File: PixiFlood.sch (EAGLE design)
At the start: 36 parts, among them IC1 WS2811-SOP8, IC2 78L05Z, T1 2N3904, T2 2N3904, T3 2N3904, U1 PT4115B89E, U2 PT4115B89E, U3 PT4115B89E, X2 22-23-2041

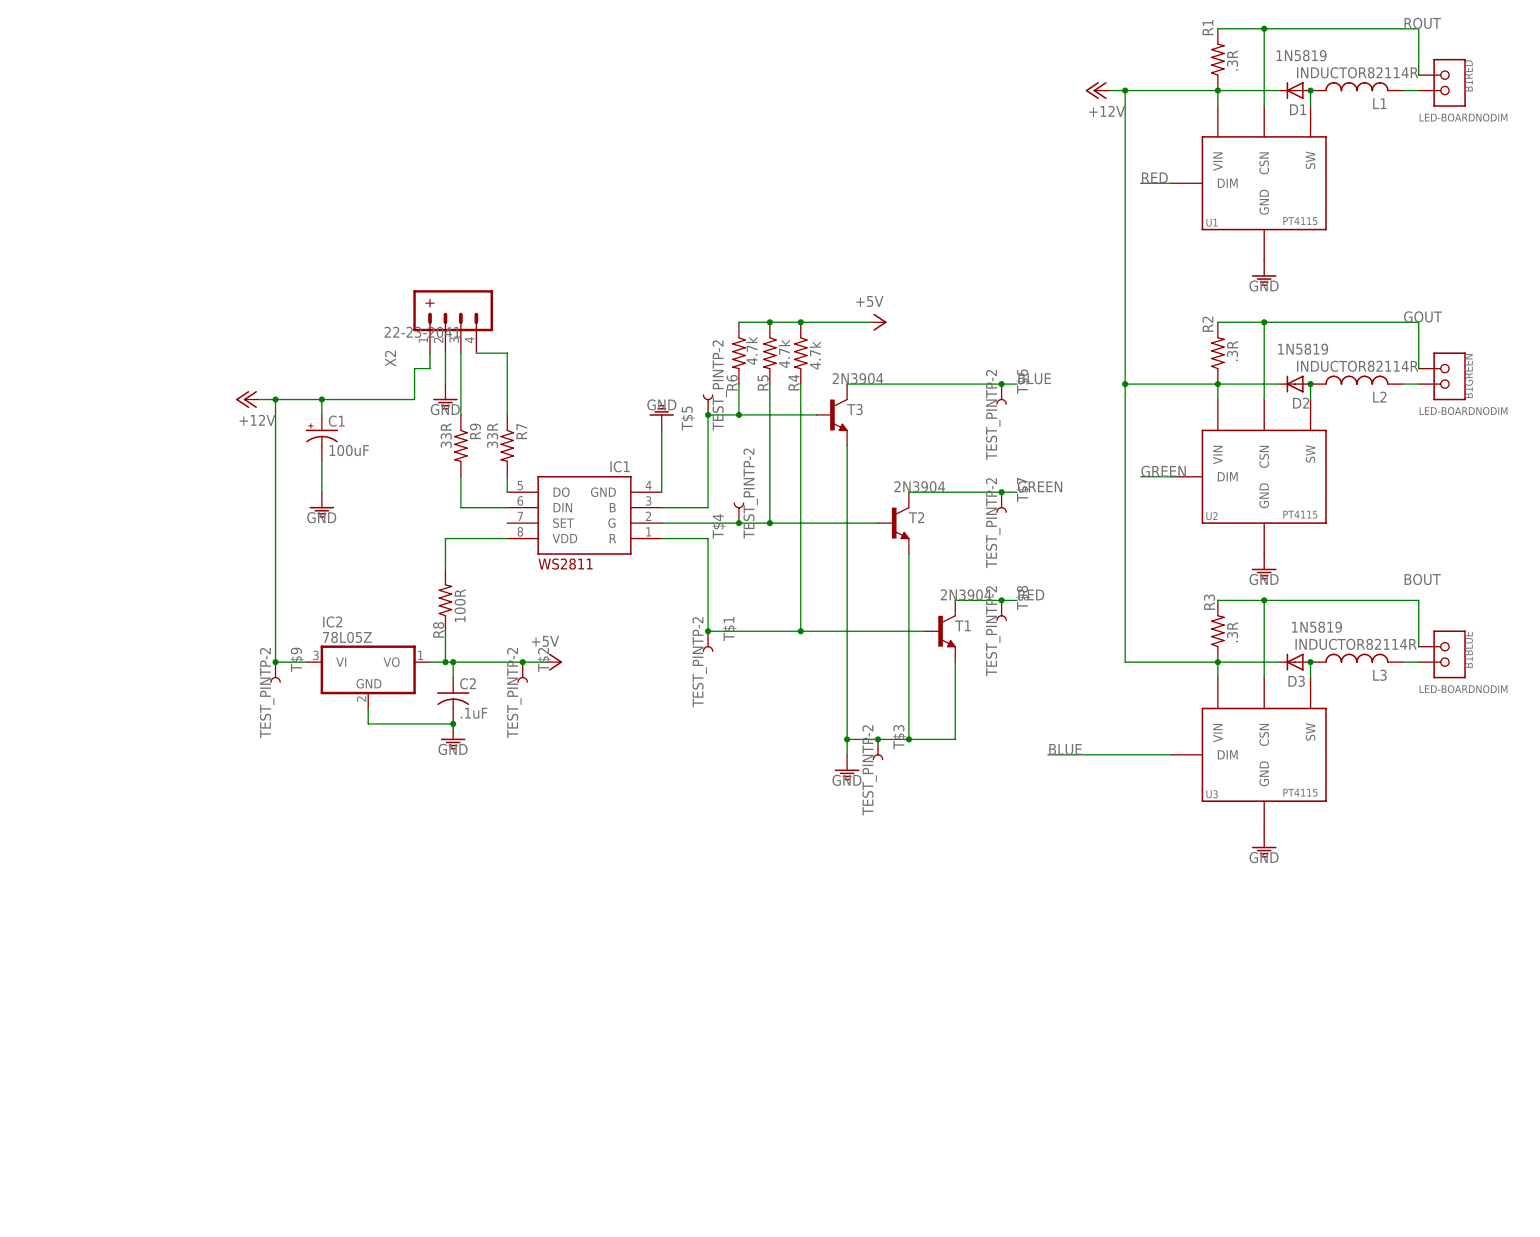
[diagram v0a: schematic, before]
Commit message: Initial Commit
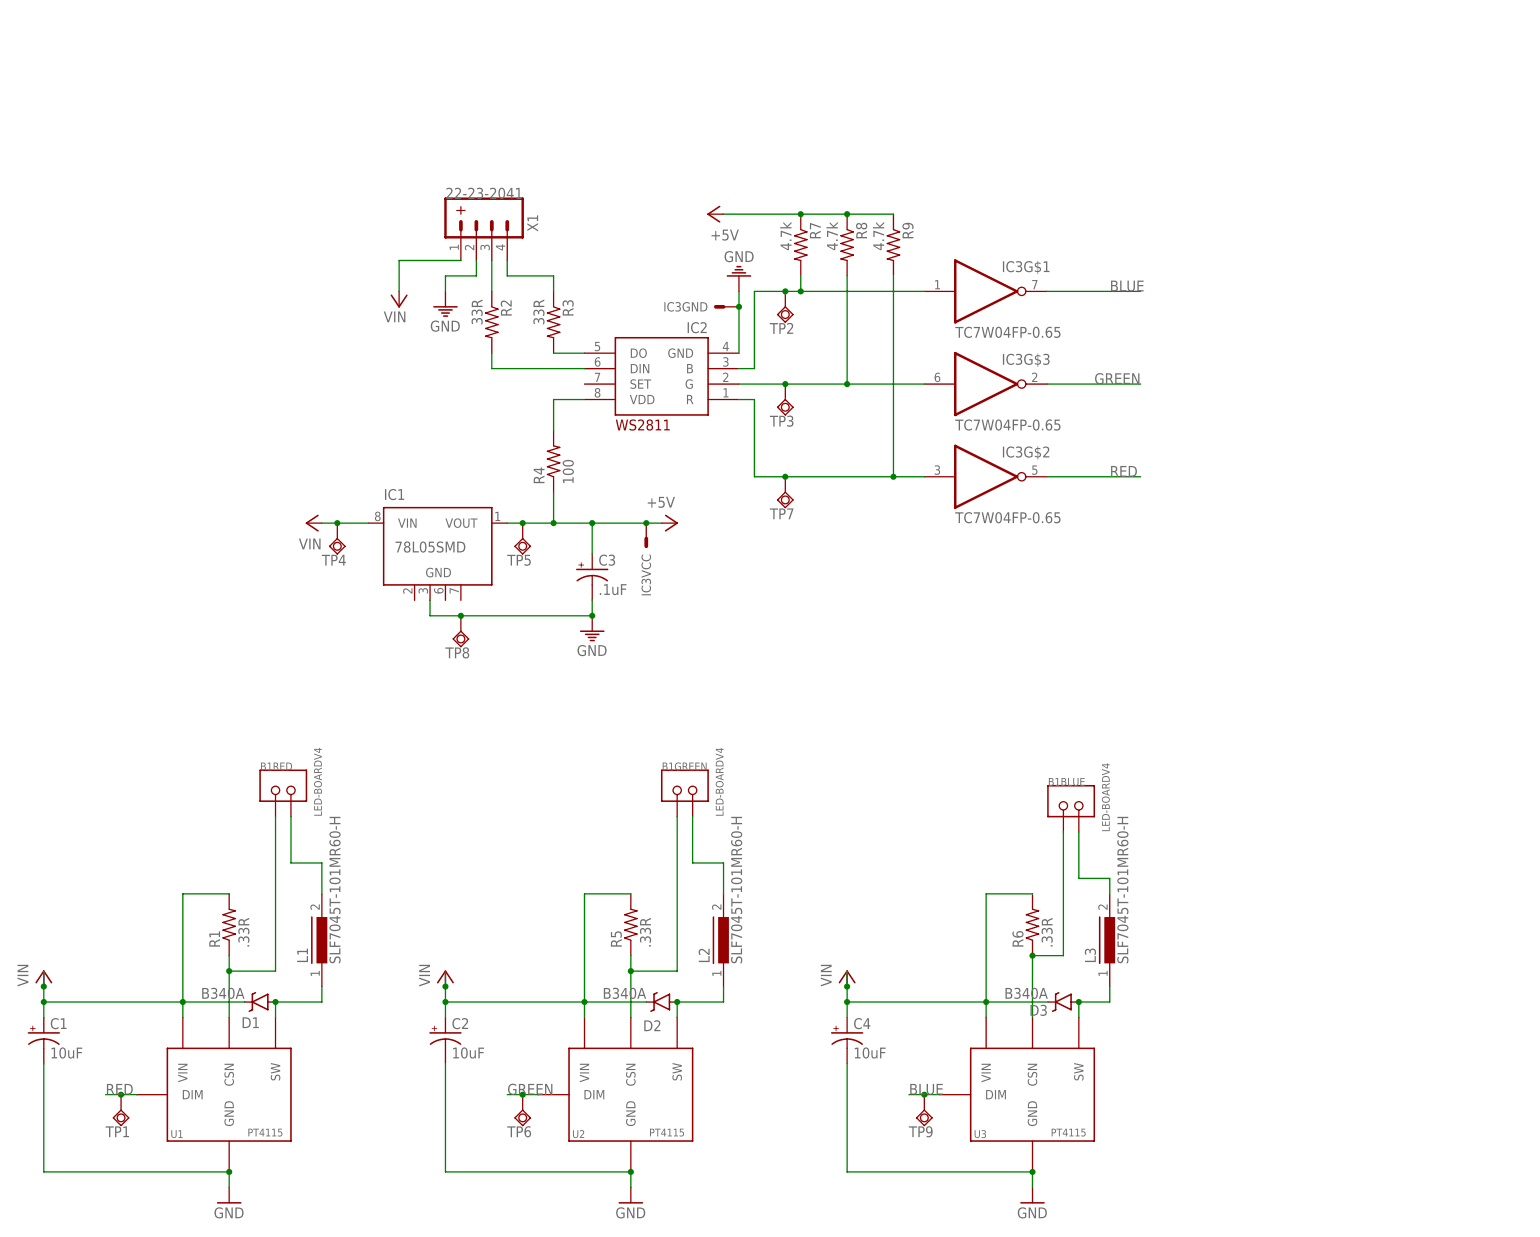
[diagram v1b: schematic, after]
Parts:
- removed T$1, T$2, T$3, T$4, T$5, T$6, T$7, T$8, T$9: TEST_PINTP-2, headers:TEST_PINTP-2
- removed T1, T2, T3: 2N3904, transistor:2N3904
- removed X2: 22-23-2041, connectors:22-23-2041
- added C3: .1uF, capacitors:CAP_POL1206
- added C4: 10uF, capacitors:CAP_POLCASE-D
- added IC3: TC7W04FP-0.65, logic:TC7W04FP-0.65
- added TP1, TP2, TP3, TP4, TP5, TP6, TP7, TP9: TPSQTP15R, testpad:TPSQTP15R
- added TP8: TPSQTP20SQ, testpad:TPSQTP20SQ
- added X1: 22-23-2041, connectors:22-23-2041
- B1: value LED-BOARDNODIM -> LED-BOARDV4; device myBoards:LED-BOARDNODIM -> special:LED-BOARDV4
- C1: value 100uF -> 10uF; device rcl:CPOL-USTT2D6L -> capacitors:CAP_POLCASE-D
- C2: value .1uF -> 10uF; device rcl:C-US050-024X044 -> capacitors:CAP_POLCASE-D
- D1, D2, D3: value 1N5819 -> B340A; device diode:DIODE-DO07 -> SparkFun-DiscreteSemi:DIODE-SCHOTTKY-B340A
- IC1: value WS2811-SOP8 -> 78L05SMD; device MyLibrary:WS2811-SOP8 -> regulators:78L05SMD
- IC2: value 78L05Z -> WS2811S; device linear:78L05Z -> drivers:WS2811S
- L1, L2, L3: value INDUCTOR82114R -> SLF7045T-101MR60-H; device rcl:INDUCTOR82114R -> inductors:SLF7045
- R1: value .3R -> .33R; device resistor:R-US_0204/7 -> resistor:R-US_R1210
- R2, R3: value .3R -> 33R; device resistor:R-US_0204/7 -> rcl:R-US_R1206
- R4: value 4.7k -> 100; device resistor:R-US_0204/7 -> rcl:R-US_R1206
- R5, R6: value 4.7k -> .33R; device resistor:R-US_0204/7 -> resistor:R-US_R1210
- R7, R9: value 33R -> 4.7k; device rcl:R-US_0204/7 -> rcl:R-US_R1206
- R8: value 100R -> 4.7k; device rcl:R-US_0204/7 -> rcl:R-US_R1206
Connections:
- removed net +12V: C1.+, D1.C, D2.C, D3.C, IC2.VI, R1.1, R2.1, R3.1, T$9.1, U1.VIN, U2.VIN, U3.VIN, X2.1
- removed net DIN-R: IC1.DIN, R9.2
- removed net DO-R: IC1.DO, R7.2
- removed net N$15: IC1.B, R6.2, T$5.1, T3.B
- removed net N$18: IC1.G, R5.2, T$4.1, T2.B
- removed net N$20: IC1.R, R4.2, T$1.1, T1.B
- new net BLU-WS: IC2.B, IC3G$1.I, R7.2, TP2.TP
- new net DIN-E: R2.1, X1.3
- new net DO-E: R3.1, X1.4
- new net GREN-WS: IC2.G, IC3G$3.I, R8.2, TP3.TP
- new net RED-WS: IC2.R, IC3G$2.I, R9.2, TP7.TP
- new net VIN: C1.+, C2.+, C4.+, D1.C, D2.C, D3.C, IC1G$1.VIN, R1.2, R5.2, R6.2, TP4.TP, U1.VIN, U2.VIN, U3.VIN, X1.1
- net +5V: now also C3.+, IC1G$1.VOUT, IC3VCC.S, R7.1, R9.1, TP5.TP; no longer C2.1, IC2.VO, R5.1, R6.1, T$2.1
- net BLUE: now also IC3G$1.O, TP9.TP; no longer T$6.1, T3.C
- net BOUT: now also R6.1; no longer R3.2
- net DIN: now also IC2.DIN, R2.2; no longer R9.1, X2.3
- net DO: now also IC2.DO, R3.2; no longer R7.1, X2.4
- net GND: now also C2.-, C3.-, C4.-, IC1G$1.GND@2, IC3GND.S, TP8.TP, X1.2; no longer C2.2, IC1.GND, T$3.1, T1.E, T2.E, T3.E, X2.2
- net GOUT: now also R5.1; no longer R2.2
- net GREEN: now also IC3G$3.O, TP6.TP; no longer T$7.1, T2.C
- net RED: now also IC3G$2.O, TP1.TP; no longer T$8.1, T1.C
- net ROUT: now also R1.1; no longer R1.2
- net VDD: now also IC2.VDD, R4.2; no longer IC1.VDD, R8.2
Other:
- moved on the sheet: B1BLUE, B1GREEN, B1RED, C1, R1, R2, R3, R4, R5, R6, R7, R8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
